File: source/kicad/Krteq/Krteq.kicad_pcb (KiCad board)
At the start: 2 copper layers, 228.6 x 116.3 mm, 263 parts, among them Q1 Q NMOS GSD, Q2 Q NMOS GSD, Q3 Q NMOS GSD, Q4 Q NMOS GSD, SW1 Switch, SW10 Switch, SW11 Switch, SW12 Switch, SW13 Switch, SW14 Switch, SW15 Switch, SW16 Switch, SW17 Switch, SW18 Switch, SW19 Switch, SW2 Switch, SW20 Switch, SW21 Switch, SW22 Switch, SW23 Switch, SW24 Switch, SW25 Switch, SW26 Switch, SW27 Switch, SW28 Switch, SW29 Switch, SW3 Switch, SW30 Switch, SW31 Switch, SW32 Switch, SW33 Switch, SW34 Switch, SW35 Switch, SW36 Switch, SW37 Switch, SW38 Switch, SW39 Switch, SW4 Switch, SW40 Switch, SW41 Switch, SW42 Switch, SW43 Switch, SW44 Switch, SW45 Switch, SW46 Switch, SW47 Switch, SW48 Switch, SW49 Switch, SW5 Switch, SW50 Switch, SW51 Switch, SW52 Switch, SW53 Switch, SW54 Switch, SW55 Switch, SW56 Switch, SW57 Switch, SW58 Switch, SW59 Switch, SW6 Switch, SW60 Switch, SW61 Switch, SW7 Switch, SW8 Switch, SW9 Switch

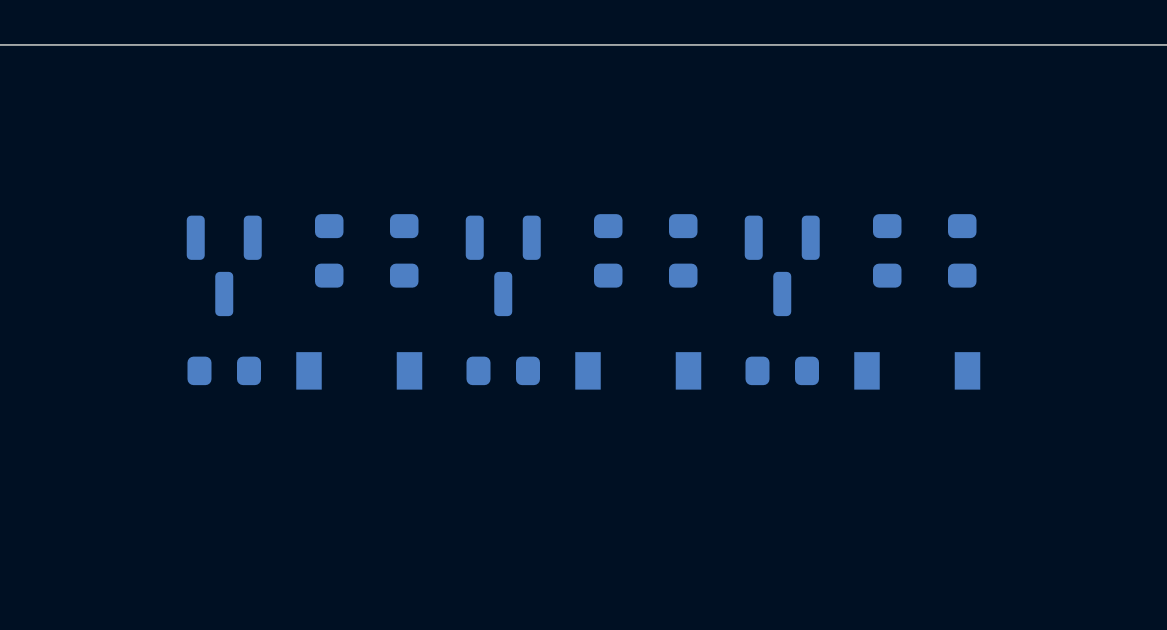
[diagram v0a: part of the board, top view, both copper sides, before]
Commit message: tweaks
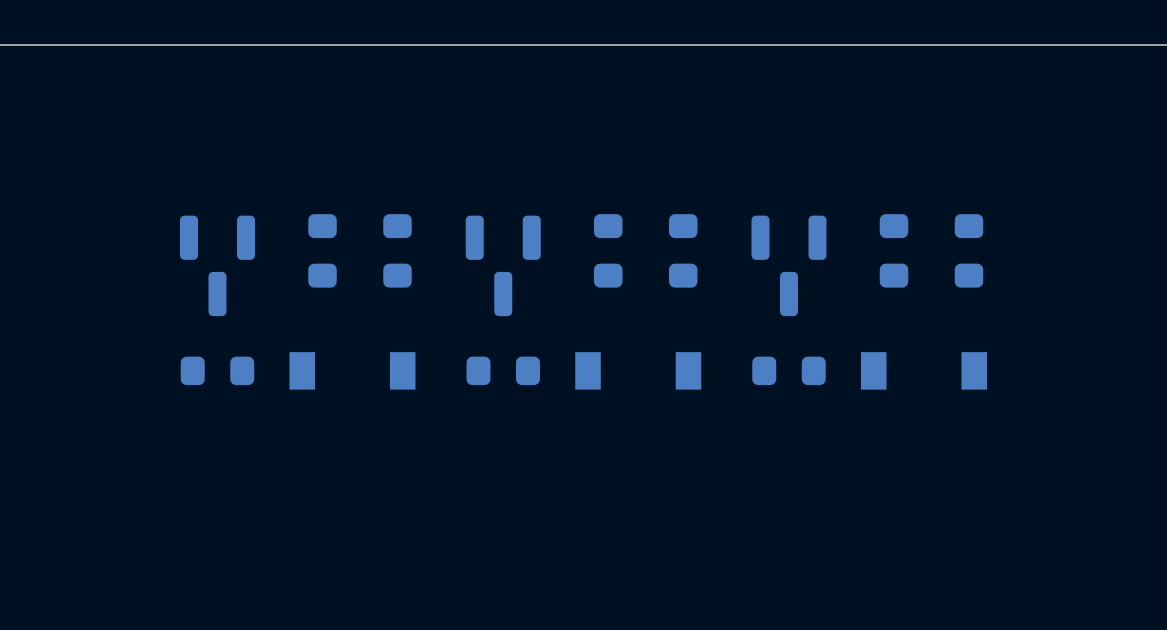
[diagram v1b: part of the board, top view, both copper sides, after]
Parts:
- moved D1 0.22 mm to (209.9, 85.7)
- moved D3 0.22 mm to (228.9, 85.7)
- moved Q1 0.22 mm to (205.4, 82.2)
- moved Q3 0.22 mm to (224.4, 82.2)
- moved R1 0.22 mm to (205.4, 85.7)
- moved R2 0.22 mm to (211.4, 81.7)
- moved R3 0.22 mm to (208.9, 81.7)
- moved R7 0.22 mm to (224.4, 85.7)
- moved R8 0.22 mm to (230.4, 81.7)
- moved R9 0.22 mm to (227.9, 81.7)
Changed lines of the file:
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@@
 	(footprint "Resistor_SMD:R_0603_1608Metric"
 		(layer "B.Cu")
-		(at 209.125 81.738625 -90)
+		(at 208.9 81.738625 -90)
 		(descr "Resistor SMD 0603 (1608 Metric), square (rectangular) end terminal, IPC-7351 nominal, (Body size source: IPC-SM-782 page 72, https://www.pcb-3d.com/wordpress/wp-content/uploads/ipc-sm-782a_amendment_1_and_2.pdf), generated with kicad-footprint-generator")
 		(tags "resistor")
@@
 	(footprint "Package_TO_SOT_SMD:SOT-23"
 		(layer "B.Cu")
-		(at 224.225 82.238625 -90)
+		(at 224.45 82.238625 -90)
 		(descr "SOT, 3 Pin (JEDEC TO-236 Var AB https://www.jedec.org/document_search?search_api_views_fulltext=TO-236), generated with kicad-footprint-generator ipc_gullwing_generator.py")
 		(tags "SOT TO_SOT_SMD")
@@
 	(footprint "Package_TO_SOT_SMD:SOT-23"
 		(layer "B.Cu")
-		(at 205.625 82.238625 -90)
+		(at 205.4 82.238625 -90)
 		(descr "SOT, 3 Pin (JEDEC TO-236 Var AB https://www.jedec.org/document_search?search_api_views_fulltext=TO-236), generated with kicad-footprint-generator ipc_gullwing_generator.py")
 		(tags "SOT TO_SOT_SMD")
@@
 	(footprint "Resistor_SMD:R_0603_1608Metric"
 		(layer "B.Cu")
-		(at 227.725 81.738625 -90)
+		(at 227.95 81.738625 -90)
 		(descr "Resistor SMD 0603 (1608 Metric), square (rectangular) end terminal, IPC-7351 nominal, (Body size source: IPC-SM-782 page 72, https://www.pcb-3d.com/wordpress/wp-content/uploads/ipc-sm-782a_amendment_1_and_2.pdf), generated with kicad-footprint-generator")
 		(tags "resistor")
@@
 	(footprint "Resistor_SMD:R_0603_1608Metric"
 		(layer "B.Cu")
-		(at 230.225 81.738625 90)
+		(at 230.45 81.738625 90)
 		(descr "Resistor SMD 0603 (1608 Metric), square (rectangular) end terminal, IPC-7351 nominal, (Body size source: IPC-SM-782 page 72, https://www.pcb-3d.com/wordpress/wp-content/uploads/ipc-sm-782a_amendment_1_and_2.pdf), generated with kicad-footprint-generator")
 		(tags "resistor")
@@
 	(footprint "Resistor_SMD:R_0603_1608Metric"
 		(layer "B.Cu")
-		(at 211.625 81.738625 90)
+		(at 211.4 81.738625 90)
 		(descr "Resistor SMD 0603 (1608 Metric), square (rectangular) end terminal, IPC-7351 nominal, (Body size source: IPC-SM-782 page 72, https://www.pcb-3d.com/wordpress/wp-content/uploads/ipc-sm-782a_amendment_1_and_2.pdf), generated with kicad-footprint-generator")
 		(tags "resistor")
@@
 	(footprint "Krteq:MHT151WDT"
 		(layer "B.Cu")
-		(at 228.725 85.738625)
+		(at 228.95 85.738625)
 		(descr "-35℃~+85℃ 130° 20mA 3.65V 900mcd 95mW Frosted Yellow Lens Reverse Mount White 1206 LED Indication - Discrete ROHS")
 		(tags "diode reverse")
@@
 	(footprint "Resistor_SMD:R_0603_1608Metric"
 		(layer "B.Cu")
-		(at 205.625 85.738625 180)
+		(at 205.4 85.738625 180)
 		(descr "Resistor SMD 0603 (1608 Metric), square (rectangular) end terminal, IPC-7351 nominal, (Body size source: IPC-SM-782 page 72, https://www.pcb-3d.com/wordpress/wp-content/uploads/ipc-sm-782a_amendment_1_and_2.pdf), generated with kicad-footprint-generator")
 		(tags "resistor")
@@
 	(footprint "Resistor_SMD:R_0603_1608Metric"
 		(layer "B.Cu")
-		(at 224.225 85.738625 180)
+		(at 224.45 85.738625 180)
 		(descr "Resistor SMD 0603 (1608 Metric), square (rectangular) end terminal, IPC-7351 nominal, (Body size source: IPC-SM-782 page 72, https://www.pcb-3d.com/wordpress/wp-content/uploads/ipc-sm-782a_amendment_1_and_2.pdf), generated with kicad-footprint-generator")
 		(tags "resistor")
@@
 	(footprint "Krteq:MHT151WDT"
 		(layer "B.Cu")
-		(at 210.125 85.738625)
+		(at 209.9 85.738625)
 		(descr "-35℃~+85℃ 130° 20mA 3.65V 900mcd 95mW Frosted Yellow Lens Reverse Mount White 1206 LED Indication - Discrete ROHS")
 		(tags "diode reverse")

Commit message: pcb v1
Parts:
- A1: footprint Module:RaspberryPi_Pico_Common_THT -> Krteq:Pi Pico
- moved R11 4.07 mm to (302.5, 83.7), turned to 0 degrees
- moved R10 3.41 mm to (298.9, 83.7), turned to 180 degrees
- moved Q4 0.82 mm to (300.7, 80.1), turned to 90 degrees
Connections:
- A1 pad 1: SIG2 -> SIG1
- A1 pad 12: unconnected-(A1-GPIO9-Pad12) -> ROW5
- A1 pad 14: ROW3 -> ROW4
- A1 pad 15: ROW4 -> ROW3
- A1 pad 16: ROW5 -> ROW2
- A1 pad 17: COL10 -> BL PWM
- A1 pad 19: COL11 -> unconnected-(A1-GPIO14-Pad19)
- A1 pad 2: SIG3 -> SIG2
- A1 pad 20: BL PWM -> unconnected-(A1-GPIO15-Pad20)
- A1 pad 21: ROW0 -> COL10
- A1 pad 22: ROW1 -> COL11
- A1 pad 24: ROW2 -> ROW0
- A1 pad 25: unconnected-(A1-GPIO19-Pad25) -> ROW1
- A1 pad 4: SIG1 -> SIG3
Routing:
- net VBUS: track 0.00 -> 1668.3 mm, vias 0 -> 72
- net BL DRAIN: track 0.00 -> 1589.5 mm, vias 0 -> 76
- net ROW5: track 0.00 -> 421.7 mm, vias 0 -> 13
- net ROW4: track 0.00 -> 393.7 mm, vias 0 -> 14
- net ROW3: track 0.00 -> 355.8 mm, vias 0 -> 14
- net ROW2: track 0.00 -> 319.0 mm, vias 0 -> 14
- net COL0: track 0.00 -> 261.2 mm
- net ROW1: track 0.00 -> 242.7 mm, vias 0 -> 12
- net COL1: track 0.00 -> 239.0 mm
- net ROW0: track 0.00 -> 229.9 mm, vias 0 -> 4
- net COL2: track 0.00 -> 222.5 mm
- net COL3: track 0.00 -> 209.6 mm
- net COL4: track 0.00 -> 192.4 mm
- net COL6: track 0.00 -> 157.4 mm
- net COL5: track 0.00 -> 152.0 mm
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- added copper zone on B.Cu, net GND
- added copper zone on F.Cu, net GND
